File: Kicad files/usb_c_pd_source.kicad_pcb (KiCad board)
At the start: 2 copper layers, 75.7 x 42.4 mm, 53 parts, among them J1 Barrel_Jack, J2 Lab_supply, J3 Serial Wire, J4 USB4151-GF-C, Q1 DMP3013SFV-7, Q2 DMP3013SFV-7, Q3 DMP3013SFV-7, U1 TPS560430X3FDBVR, U2 TPS56837HRPAR, U3 STM32G030F6Px, U4 STUSB4710AQ1TR

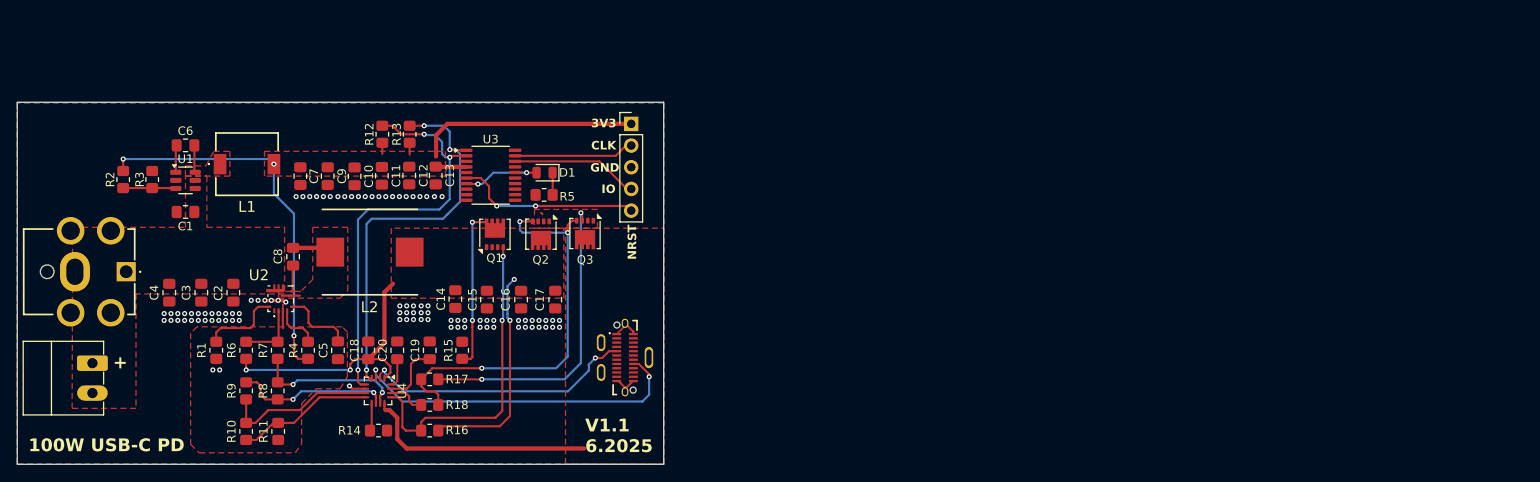
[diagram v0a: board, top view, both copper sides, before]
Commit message: Add files via upload
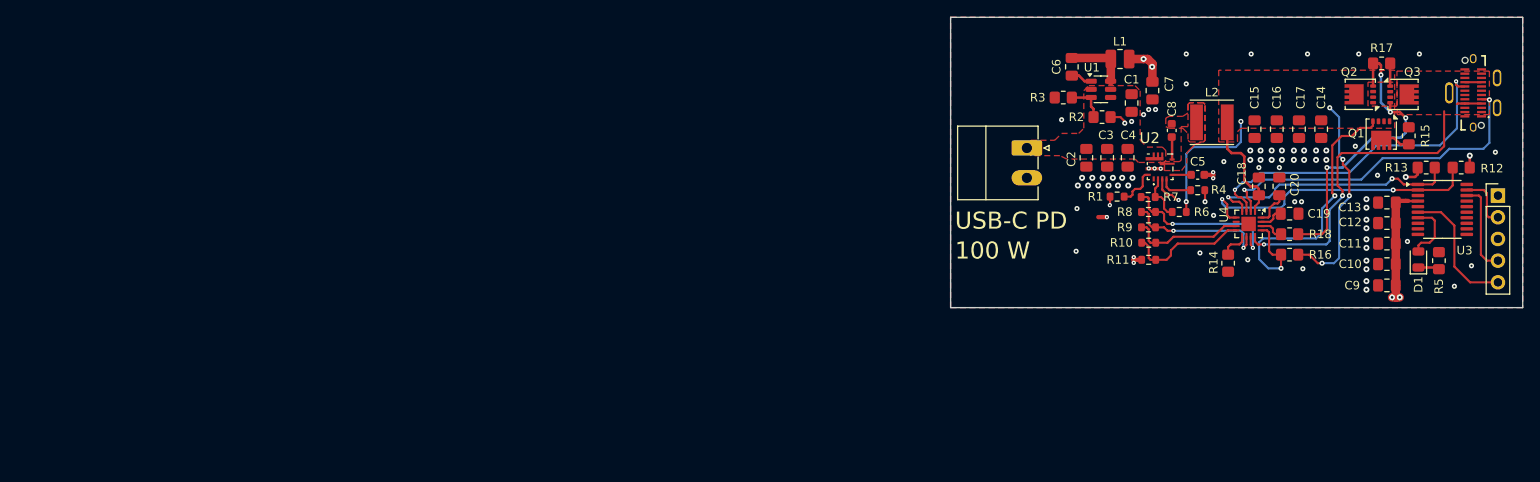
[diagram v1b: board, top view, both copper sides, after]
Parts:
- removed J1: Barrel_Jack, footprints:PJ106AHTR
- removed NT1: NetTie_2, NetTie:NetTie-2_SMD_Pad0.5mm
- added NT2: NetTie_2, NetTie:NetTie-2_SMD_Pad0.5mm, F.Cu at (191.8, 122.4)
- C5, C8: footprint Capacitor_SMD:C_0805_2012Metric_Pad1.18x1.45mm_HandSolder -> Capacitor_SMD:C_0603_1608Metric
- C9: value 10u -> 4u7
- L1: value 12u -> 6u8; footprint footprints:SRR0735A120M -> Inductor_SMD:L_1008_2520Metric
- L2: footprint footprints:INDPM112100X400N -> Inductor_SMD:L_Taiyo-Yuden_MD-5050
- R1, R10, R11, R4, R6, R7, R8, R9: footprint Resistor_SMD:R_0805_2012Metric_Pad1.20x1.40mm_HandSolder -> Resistor_SMD:R_0603_1608Metric
- U1: value TPS560430X3FDBVR -> TPS560430YFDBVR
- moved R12 126.4 mm to (233.8, 116.6), turned to 0 degrees
- moved C9 124.7 mm to (225.1, 130.4), turned to 180 degrees
- moved C10 121.3 mm to (225.1, 127.9), turned to 180 degrees
- moved R13 119.1 mm to (229.7, 116.6), turned to 180 degrees
- moved C11 118.0 mm to (225.1, 125.5), turned to 180 degrees
- moved R17 117.5 mm to (224.5, 104.4)
- moved R2 114.9 mm to (191.7, 110.7), turned to 180 degrees
- moved C12 114.6 mm to (225.1, 123.1), turned to 180 degrees
- moved R15 113.7 mm to (227.7, 112.9)
- moved C4 113.3 mm to (194.7, 115.5)
- moved J2 112.3 mm to (182.9, 114.3)
- moved C1 111.5 mm to (195.2, 109.0), turned to -90 degrees
- moved U3 111.5 mm to (231.6, 121.5)
- moved C13 111.4 mm to (225.1, 120.7), turned to 180 degrees
- moved R6 110.5 mm to (200.8, 121.8), turned to 180 degrees
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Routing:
- net +3V3: track 76.7 -> 27.7 mm, vias 3 -> 8
- net /CMN_SRC: track 36.1 -> 2.66 mm, vias 2 -> 0
- net Net-(Q1-D): track 20.2 -> 3.53 mm, vias 2 -> 0
- net /SCL: track 46.8 -> 30.2 mm, vias 3 -> 2
- net /VBUS: track 27.5 -> 42.3 mm, vias 0 -> 2
- net /SDA: track 49.0 -> 34.7 mm, vias 3 -> 2
- net Net-(Q2-G): track 47.6 -> 36.3 mm, vias 3 -> 4
- net GND: track 9.24 -> 0.00 mm, vias 96 -> 69
- net /CC1: track 32.0 -> 39.8 mm
- net /SW_CLK: track 14.1 -> 6.50 mm
- net Net-(U2-SS): track 8.51 -> 2.22 mm
- net /NRST: track 21.7 -> 15.6 mm, vias 2 -> 0
- net AGND: track 2.03 -> 8.01 mm, vias 0 -> 7
- net /L_IN: track 5.96 -> 0.00 mm
- net Net-(U4-SEL_PDO3): track 18.2 -> 13.4 mm
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- added copper zone on In2.Cu, net +3V3
- added copper zone on In1.Cu, net AGND
- added copper zone on In1.Cu, net GND
- removed copper zone on F.Cu, net +3V3
- removed copper zone on F.Cu, net /L2_IN
- removed copper zone on F.Cu, net AGND
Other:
- board size 75.7 x 42.4 mm -> 67 x 34 mm
- copper layers 2 -> 4
- board text added: "100 W"
- board text added: "USB-C PD"
- board text removed: "+"
- board text removed: "100W USB-C PD"
- board text removed: "3V3"
- board text removed: "CLK"
- board text removed: "GND"
- board text removed: "IO"
- board text removed: "NRST"
- board text removed: "V1.1 6.2025"
